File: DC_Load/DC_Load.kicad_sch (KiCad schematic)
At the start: 84 parts, among them J1 Conn_01x08_Pin, J2 Conn_01x02_Pin, J3 Conn_01x06_Pin, SW1 RotaryEncoder_Switch, U1 MCP6034, U10 L7812, U11 AT90CAN64-16A, U12 TL431LP, U15 MCP3422, U2 MCP2551-I-SN, U4 NX3L4051PW_118, U5 MCP6034, U7 MCP6034, U8 MCP6034, U9 L7805, Y1 Crystal

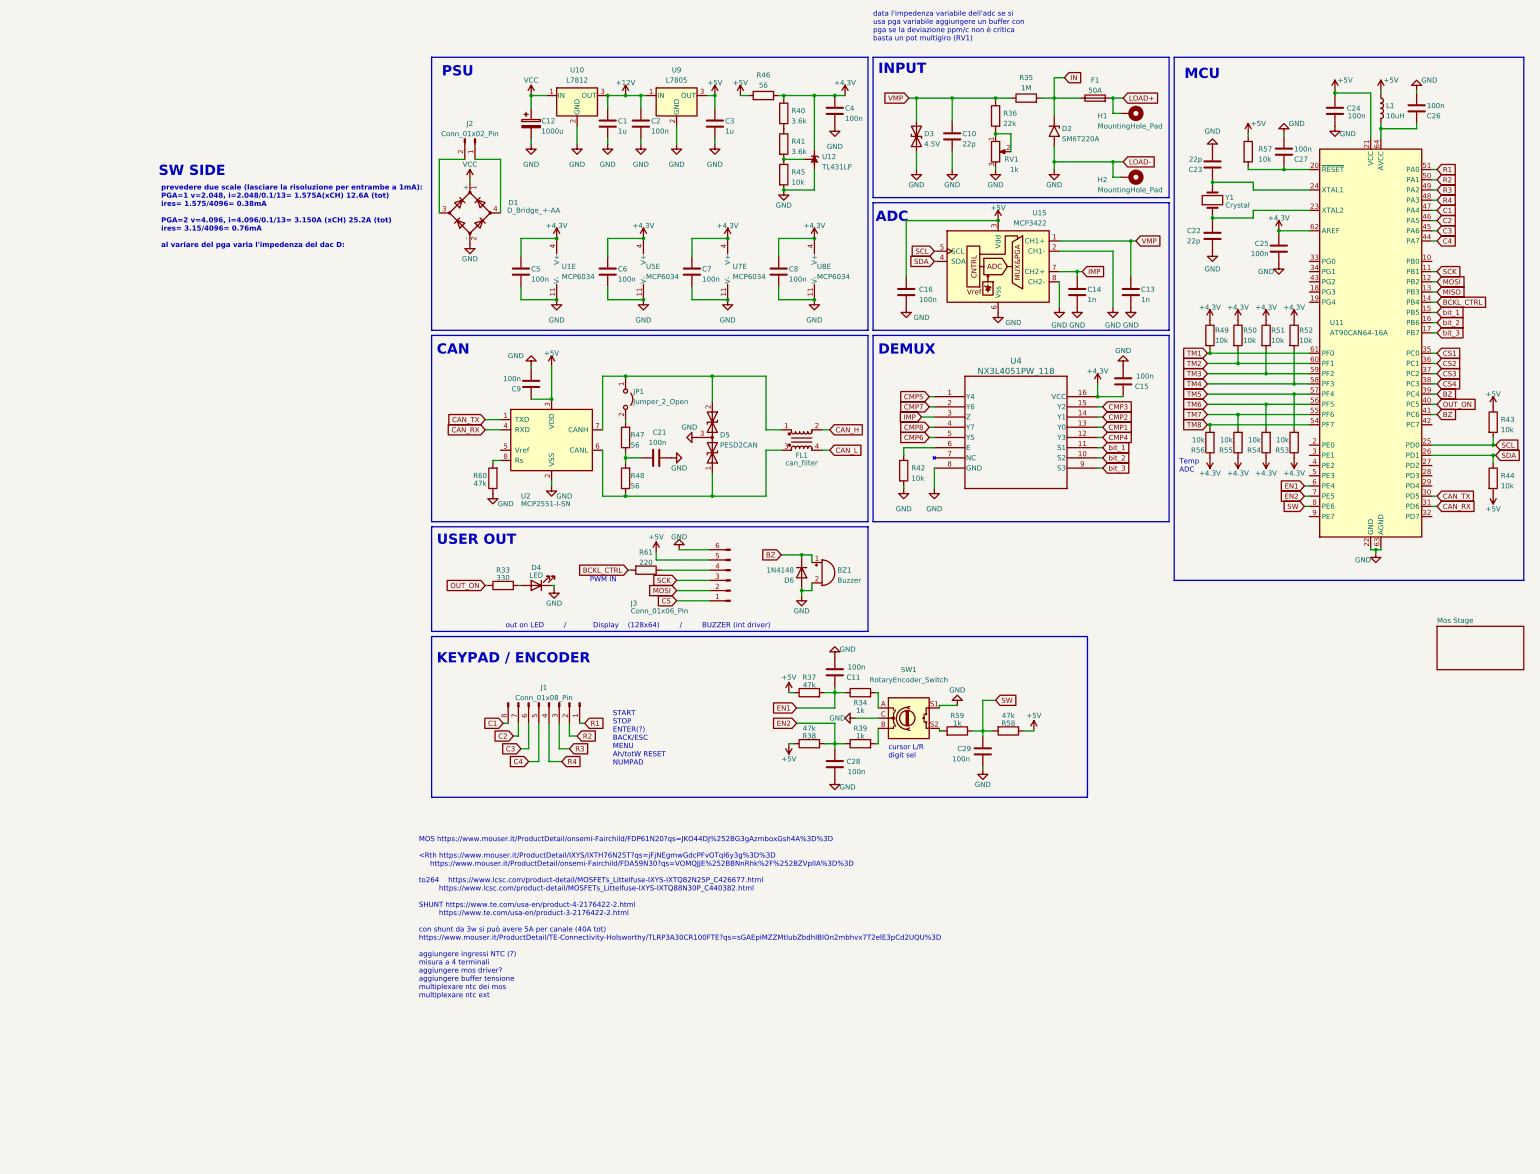
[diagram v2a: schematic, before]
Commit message: Add files via upload
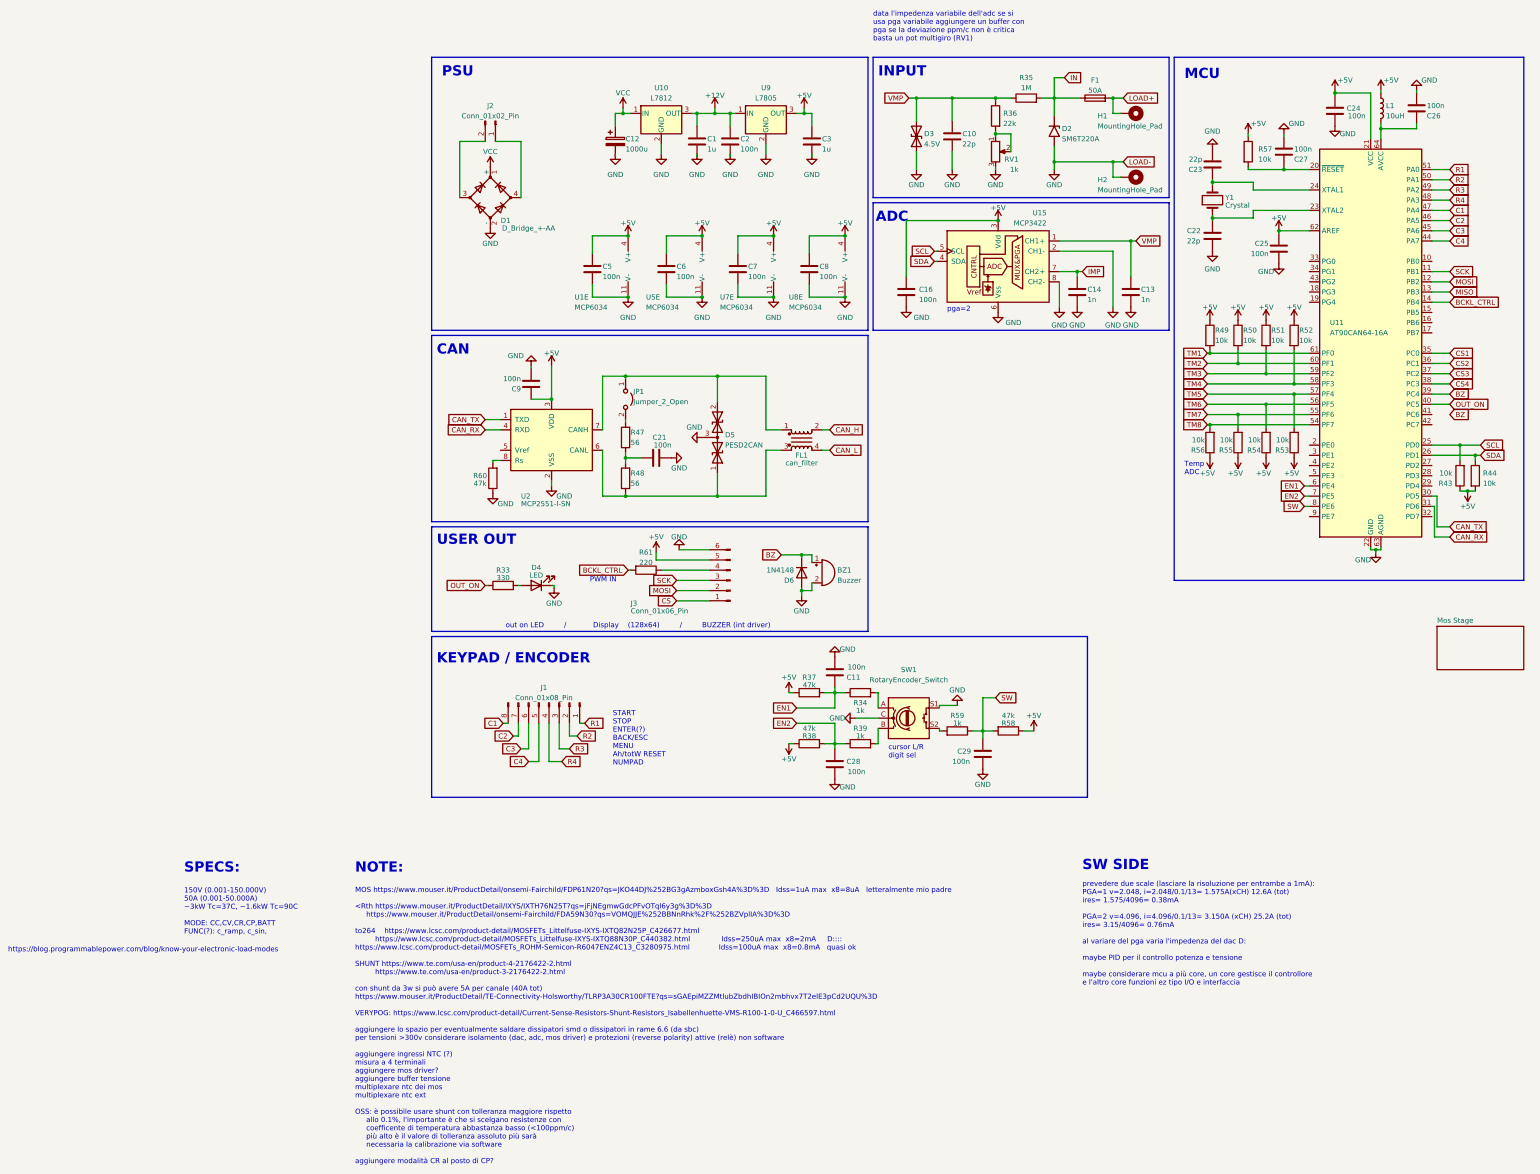
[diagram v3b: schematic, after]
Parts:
- removed C15, C4: 100n, symbol Device:C
- removed R40, R41: 3.6k, symbol Device:R
- removed R42, R45: 10k, symbol Device:R
- removed R46: 56, symbol Device:R
- removed U12: TL431LP, Package_TO_SOT_THT:TO-92_Inline, symbol Reference_Voltage:TL431LP
- removed U4: NX3L4051PW_118, TSSOP16_NXP, symbol NX3L4051:NX3L4051PW_118
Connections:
- net +4V is gone; now on net +5V: C25.1, C5.1, C6.1, C7.1, C8.1, R49.1, R50.1, R51.1, R52.1, R53.1, R54.1, R55.1, R56.1, U1.4 (V+), U11.62 (AREF), U5.4 (V+), U7.4 (V+), U8.4 (V+)
- net BZ: no longer U11.41 (PC6)
- net bit_1: no longer names the net of U11.15 (PB5)
- net bit_2: no longer names the net of U11.16 (PB6)
- net bit_3: no longer names the net of U11.17 (PB7)
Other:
- note added: "150V (0.001-150.000V) 50A (0.001-50.000A) ~3kW Tc=37C, ~1.6kW Tc=90C MODE: CC,CV,CR,CP,BATT FUNC(?): c_ramp, c_sin,"
- note added: "MOS https://www.mouser.it/ProductDetail/onsemi-Fairchild/FDP61N20?qs=JKO44DJ%252BG3gAzmboxGsh4A%3D%3D Idss=1uA max x8=8uA letteralmente mio padre <Rth https://www.mouser.it/ProductDetail/IXYS/IXTH76N25T?qs=jFjNEgmwGdcPFvOTql6y3g%3D%3D https://www.mouser.it/ProductDetail/onsemi-Fairchild/FDA59N30?qs=VOMQJJE%252BBNnRhk%2F%252BZVplIA%3D%3D to264 https://www.lcsc.com/product-detail/MOSFETs_Littelfuse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"
- note added: "NOTE:"
- note added: "SPECS:"
- note added: "https://blog.programmablepower.com/blog/know-your-electronic-load-modes"
- note added: "pga=2"
- note added: "prevedere due scale (lasciare la risoluzione per entrambe a 1mA): PGA=1 v=2.048, i=2.048/0.1/13= 1.575A(xCH) 12.6A (tot) ires= 1.575/4096= 0.38mA PGA=2 v=4.096, i=4.096/0.1/13= 3.150A (xCH) 25.2A (tot) ires= 3.15/4096= 0.76mA al variare del pga varia l'impedenza del dac D: maybe PID per il controllo potenza e tensione maybe considerare mcu a più core, un core gestisce il controllore e l'altro cor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"
- note removed: "DEMUX"
- note removed: "MOS https://www.mouser.it/ProductDetail/onsemi-Fairchild/FDP61N20?qs=JKO44DJ%252BG3gAzmboxGsh4A%3D%3D <Rth https://www.mouser.it/ProductDetail/IXYS/IXTH76N25T?qs=jFjNEgmwGdcPFvOTql6y3g%3D%3D https://www.mouser.it/ProductDetail/onsemi-Fairchild/FDA59N30?qs=VOMQJJE%252BBNnRhk%2F%252BZVplIA%3D%3D to264 https://www.lcsc.com/product-detail/MOSFETs_Littelfuse-IXYS-IXTQ82N25P_C426677.html https://www.lc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"
- note removed: "prevedere due scale (lasciare la risoluzione per entrambe a 1mA): PGA=1 v=2.048, i=2.048/0.1/13= 1.575A(xCH) 12.6A (tot) ires= 1.575/4096= 0.38mA PGA=2 v=4.096, i=4.096/0.1/13= 3.150A (xCH) 25.2A (tot) ires= 3.15/4096= 0.76mA al variare del pga varia l'impedenza del dac D:"
- moved on the sheet: C1, C12, C2, C29, C3, C5, C6, C7, C8, D1, D5, J2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
